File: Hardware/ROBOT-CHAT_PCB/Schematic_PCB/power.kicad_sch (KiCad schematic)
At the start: 15 parts, among them J5 Conn_01x02

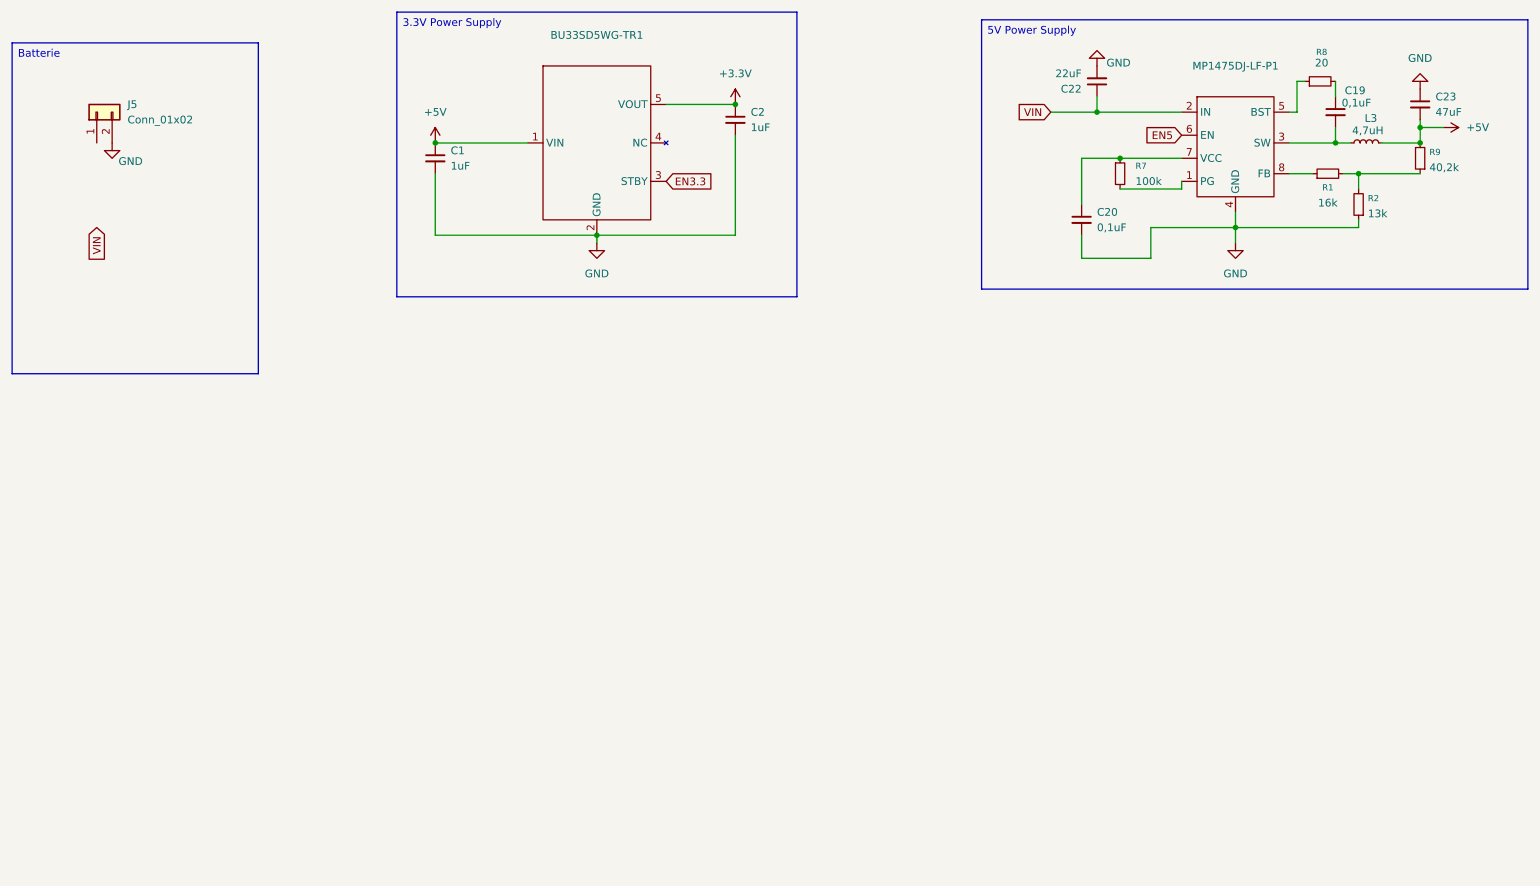
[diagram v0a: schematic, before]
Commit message: Merge PCB v3
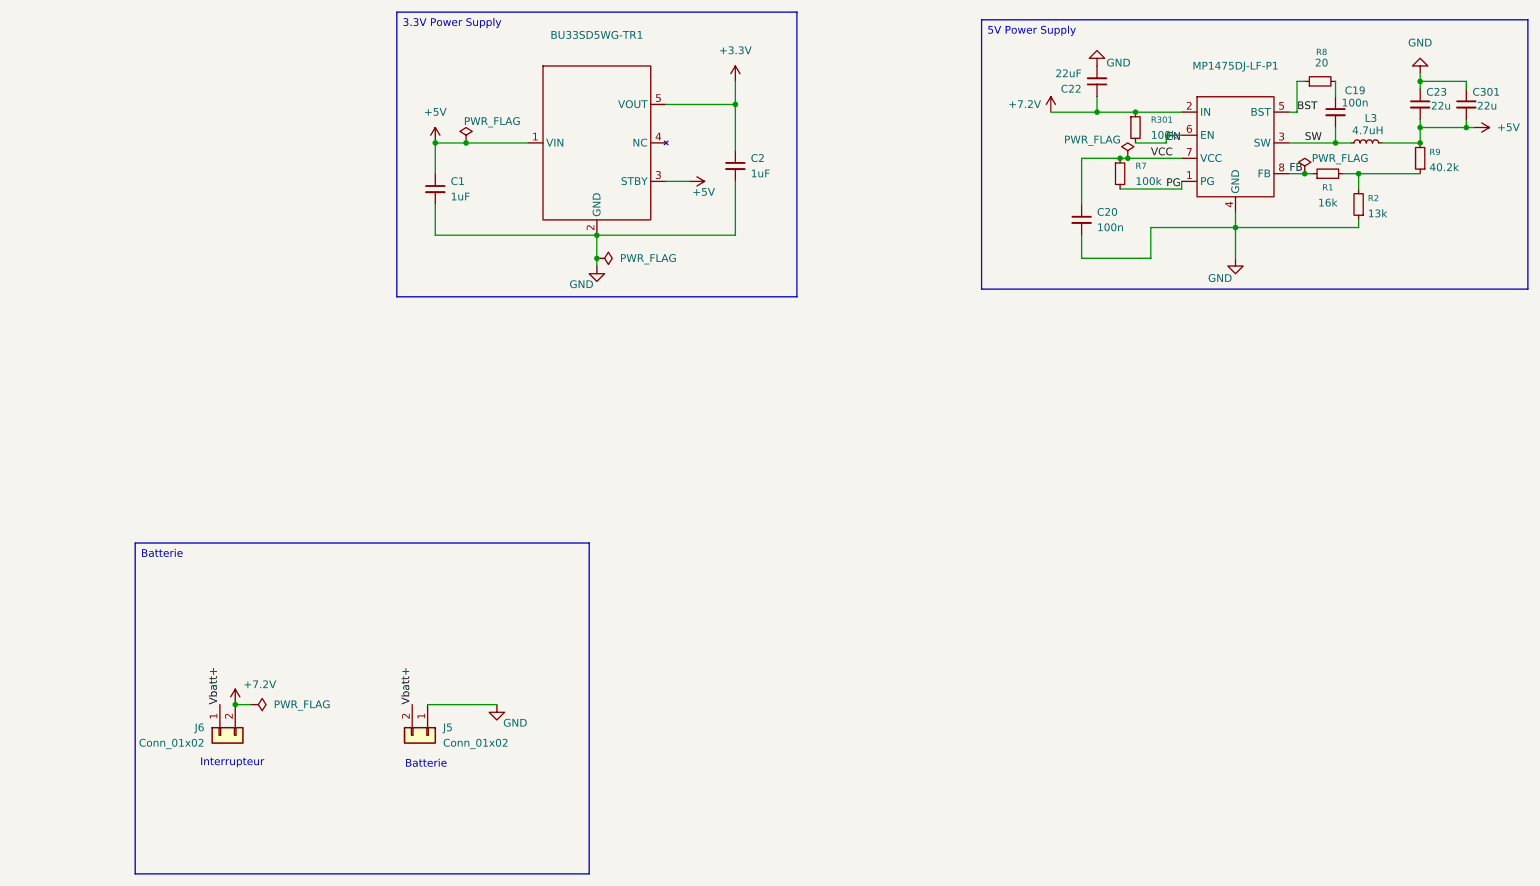
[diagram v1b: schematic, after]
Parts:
- added C301: 22u, Capacitor_SMD:C_0805_2012Metric, symbol Device:C_Small
- added J6: Conn_01x02, Connector_JST:JST_PH_B2B-PH-K_1x02_P2.00mm_Vertical, symbol Connector_Generic:Conn_01x02
- added R301: 100k, Resistor_SMD:R_0402_1005Metric, symbol Device:R_Small
- BU33SD5WG-TR1: footprint BU33SD5WG-TR:BU33SD5WG-TR -> Package_TO_SOT_SMD:SOT-23-5
- C1, C2: footprint (none) -> Capacitor_SMD:C_0603_1608Metric
- C19, C20: value 0,1uF -> 100n; footprint (none) -> Capacitor_SMD:C_0402_1005Metric
- C22: footprint (none) -> Capacitor_SMD:C_0805_2012Metric
- C23: value 47uF -> 22u; footprint (none) -> Capacitor_SMD:C_0805_2012Metric
- J5: footprint (none) -> Connector_JST:JST_PH_B2B-PH-K_1x02_P2.00mm_Vertical
- L3: value 4,7uH -> 4.7uH; footprint (none) -> Bobine_74404054068:Bobine_74404054068
- R1, R2, R7, R8: footprint (none) -> Resistor_SMD:R_0402_1005Metric
- R9: value 40,2k -> 40.2k; footprint (none) -> Resistor_SMD:R_0402_1005Metric
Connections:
- net EN3.3 is gone; now on net +5V: BU33SD5WG-TR1.3 (STBY)
- net +5V: now also C301.2
- net GND: now also J5.1 (Pin_1), C301.1; no longer J5.2 (Pin_2)
- net VCC: now reaches C20.1, MP1475DJ-LF-P1.7 (VCC), R7.1
- net PG: now reaches MP1475DJ-LF-P1.1 (PG), R7.2
- net SW: now reaches C19.2, L3.1, MP1475DJ-LF-P1.3 (SW)
- net BST: now reaches MP1475DJ-LF-P1.5 (BST), R8.1
- net FB: now reaches MP1475DJ-LF-P1.8 (FB), R1.1
- net EN5 renamed EN
- net EN: now also R301.2
- net VIN renamed +7.2V
- net +7.2V: now also J6.2 (Pin_2), R301.1
- new net Vbatt+: J5.2 (Pin_2), J6.1 (Pin_1)
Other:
- note added: "Batterie"
- note added: "Interrupteur"
- moved on the sheet: C1, C2
